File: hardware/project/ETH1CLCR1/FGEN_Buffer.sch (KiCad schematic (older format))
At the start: 45 parts, among them K1201 UMS05-1A80-75D, K1202 UMS05-1A80-75D, K1203 UMS05-1A80-75D, K1204 UMS05-1A80-75D, Q1201 MMBT4401L, Q1202 MMBT4403L, Q1203 BC847W, Q1204 BC847W, Q1205 BC847W, Q1206 BC847W, U1201 LT1468, U1202 TL072

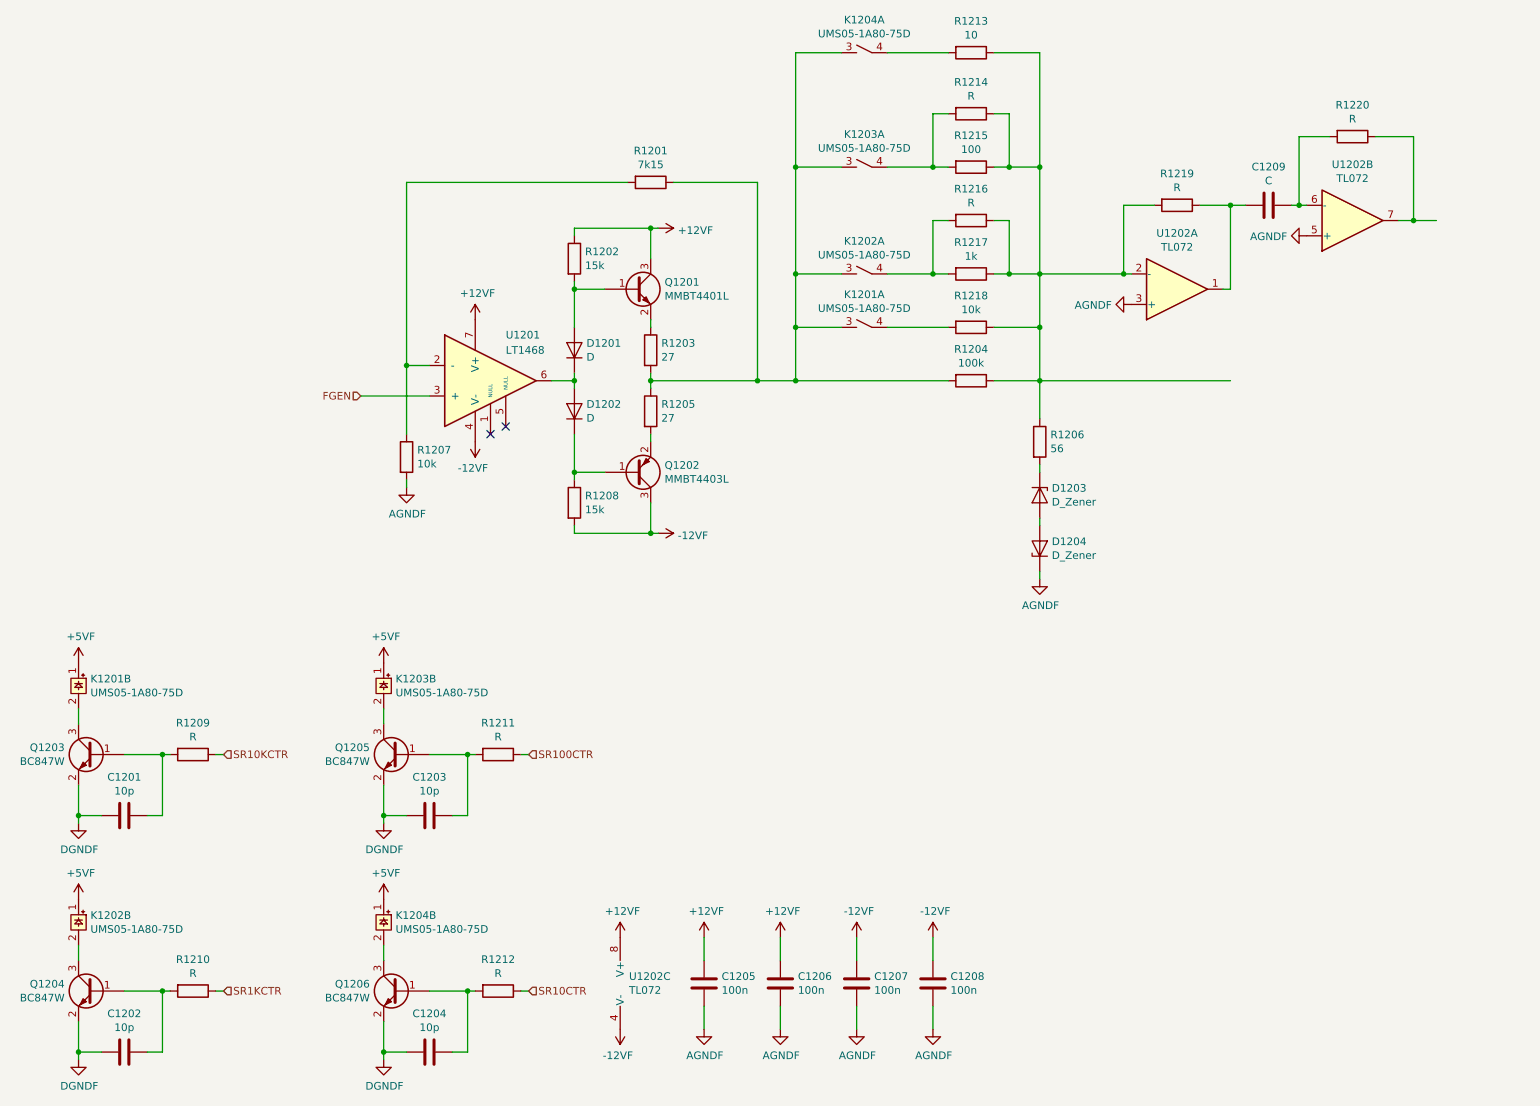
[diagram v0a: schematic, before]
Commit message: Schematic design
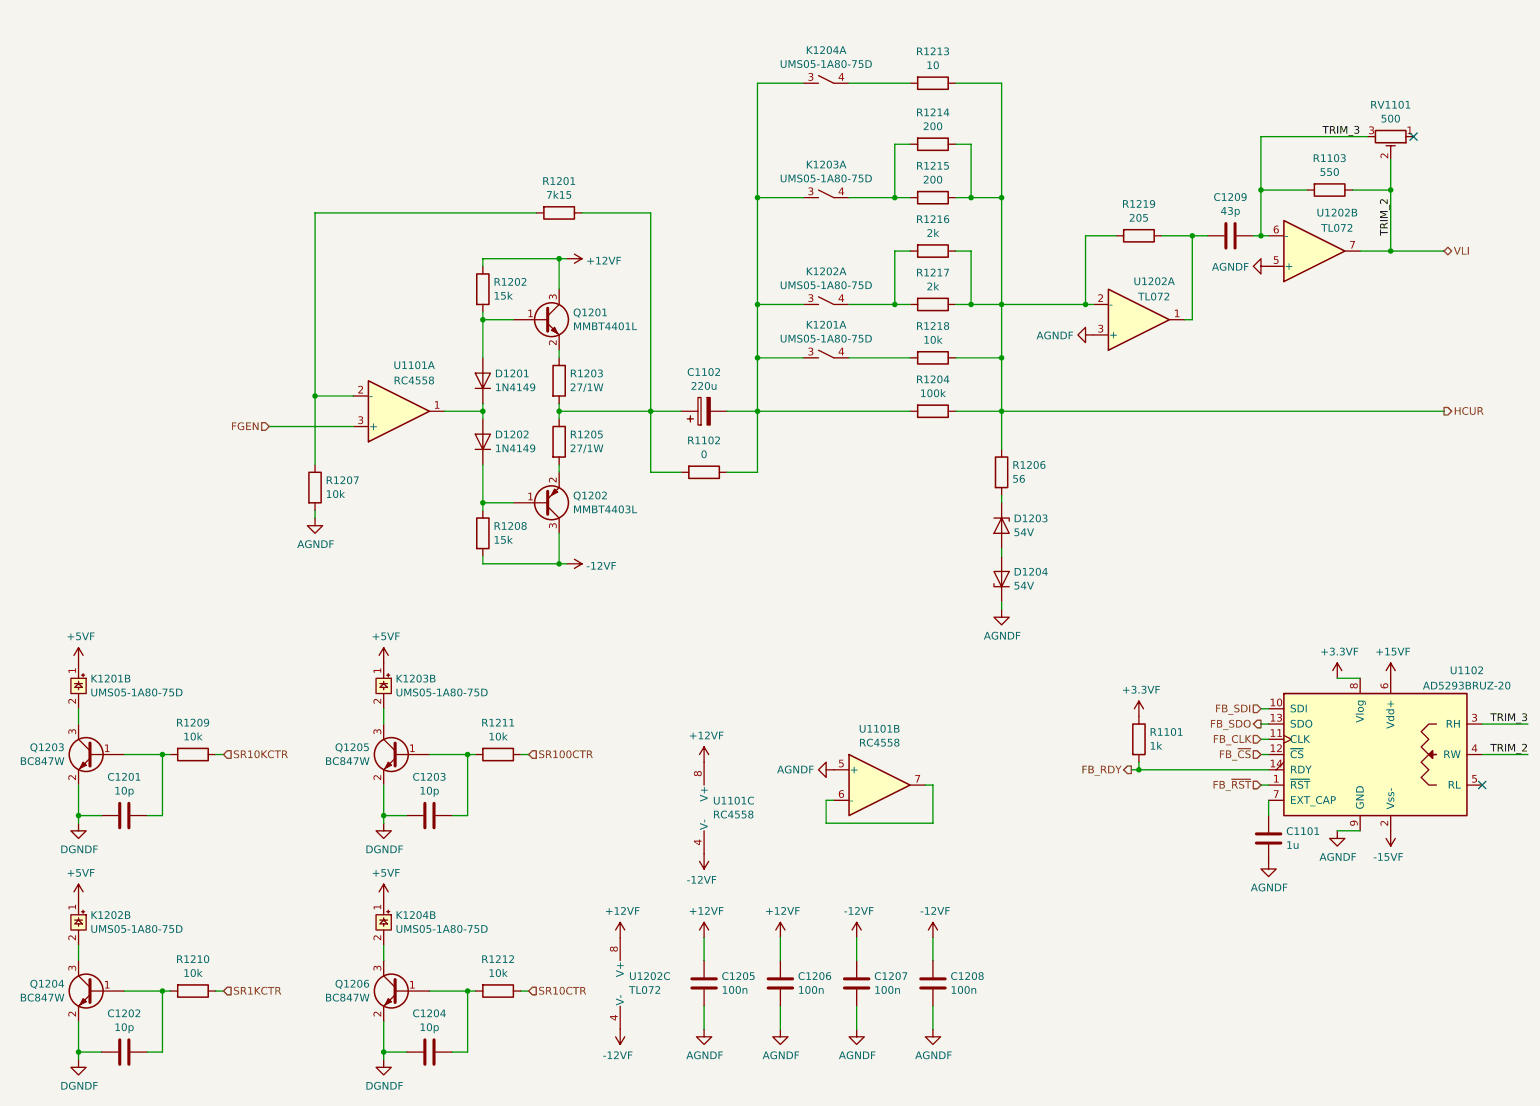
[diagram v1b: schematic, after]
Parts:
- removed R1220: R, symbol Device:R
- removed U1201: LT1468, Package_SO:SSOP-8_3.9x5.05mm_P1.27mm, symbol ETH1CLCR1:LT1468
- added C1101: 1u, symbol Device:C
- added C1102: 220u, symbol Device:CP
- added R1101: 1k, Resistor_SMD:R_0603_1608Metric_Pad1.05x0.95mm_HandSolder, symbol Device:R
- added R1102: 0, Resistor_SMD:R_0603_1608Metric_Pad1.05x0.95mm_HandSolder, symbol Device:R
- added R1103: 550, Resistor_SMD:R_0603_1608Metric_Pad1.05x0.95mm_HandSolder, symbol Device:R
- added RV1101: 500, Resistor_SMD:R_0603_1608Metric_Pad1.05x0.95mm_HandSolder, symbol Device:R_POT_TRIM
- added U1101: RC4558, symbol Amplifier_Operational:RC4558
- added U1102: AD5293BRUZ-20, Package_SO:TSSOP-14_4.4x5mm_P0.65mm, symbol Potentiometer_Digital:AD5293
- C1201, C1202, C1203, C1204, C1205, C1206, C1207, C1208: footprint (none) -> Capacitor_SMD:C_0603_1608Metric_Pad1.05x0.95mm_HandSolder
- C1209: value C -> 43p; footprint (none) -> Capacitor_SMD:C_0603_1608Metric_Pad1.05x0.95mm_HandSolder
- D1201, D1202: value D -> 1N4149
- D1203, D1204: value D_Zener -> 54V
- R1201, R1202, R1206, R1207, R1208, R1213, R1218: footprint (none) -> Resistor_SMD:R_0603_1608Metric_Pad1.05x0.95mm_HandSolder
- R1203, R1205: value 27 -> 27/1W
- R1209, R1210, R1211, R1212: value R -> 10k; footprint (none) -> Resistor_SMD:R_0603_1608Metric_Pad1.05x0.95mm_HandSolder
- R1214: value R -> 200; footprint (none) -> Resistor_SMD:R_0603_1608Metric_Pad1.05x0.95mm_HandSolder
- R1215: value 100 -> 200; footprint (none) -> Resistor_SMD:R_0603_1608Metric_Pad1.05x0.95mm_HandSolder
- R1216: value R -> 2k; footprint (none) -> Resistor_SMD:R_0603_1608Metric_Pad1.05x0.95mm_HandSolder
- R1217: value 1k -> 2k; footprint (none) -> Resistor_SMD:R_0603_1608Metric_Pad1.05x0.95mm_HandSolder
- R1219: value R -> 205; footprint (none) -> Resistor_SMD:R_0603_1608Metric_Pad1.05x0.95mm_HandSolder
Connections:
- net +12VF: now also U1101.8 (V+)
- net -12VF: now also U1101.4 (V-)
- net AGNDF: now also C1101.2, U1101.5 (+), U1102.9 (GND)
- net FGEN: now also U1101.3 (+)
- net HCUR: now reaches R1204.1, R1206.1, R1213.1, R1214.1, R1215.1, R1216.1, R1217.1, R1218.1, R1219.2, U1202.2 (-)
- net TRIM_3: now reaches C1209.1, U1202.6 (-)
- net TRIM_3: now also R1103.2, RV1101.3, U1102.3 (RH)
- net VLI: now reaches U1202.7
- net VLI: now also R1103.1, RV1101.2, U1102.4 (RW)
- net at K1201.3, K1202.3, K1203.3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: now also C1102.2, R1102.1; no longer R1201.1, R1203.2, R1205.1
- net at D1201.1 (K), D1202.2 (A): now also U1101.1
- net at R1201.2, R1207.1: now also U1101.2 (-)
- new net: U1101.6 (-), U1101.7
- new net: C1101.1, U1102.7 (EXT_CAP)
- new net: C1102.1, R1102.2, R1201.1, R1203.2, R1205.1
- new net +15VF: U1102.6 (Vdd+)
- new net +3.3VF: R1101.1, U1102.8 (Vlog)
- new net -15VF: U1102.2 (Vss-)
- new net FB_CLK: U1102.11 (CLK)
- new net FB_RDY: R1101.2, U1102.14 (RDY)
- new net FB_SDI: U1102.10 (SDI)
- new net FB_SDO: U1102.13 (SDO)
- new net FB_~CS: U1102.12 (~CS~)
- new net FB_~RST: U1102.1 (~RST~)
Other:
- moved on the sheet: C1209, D1201, D1202, D1203, D1204, K1201A, K1202A, K1203A, K1204A, Q1201, Q1202, R1201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
